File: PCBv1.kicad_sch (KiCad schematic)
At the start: 21 parts, among them J1 AVR-ISP-6, SW2 SW_Push_Reset, U1 ATmega32U4-A, Y1 16MHz

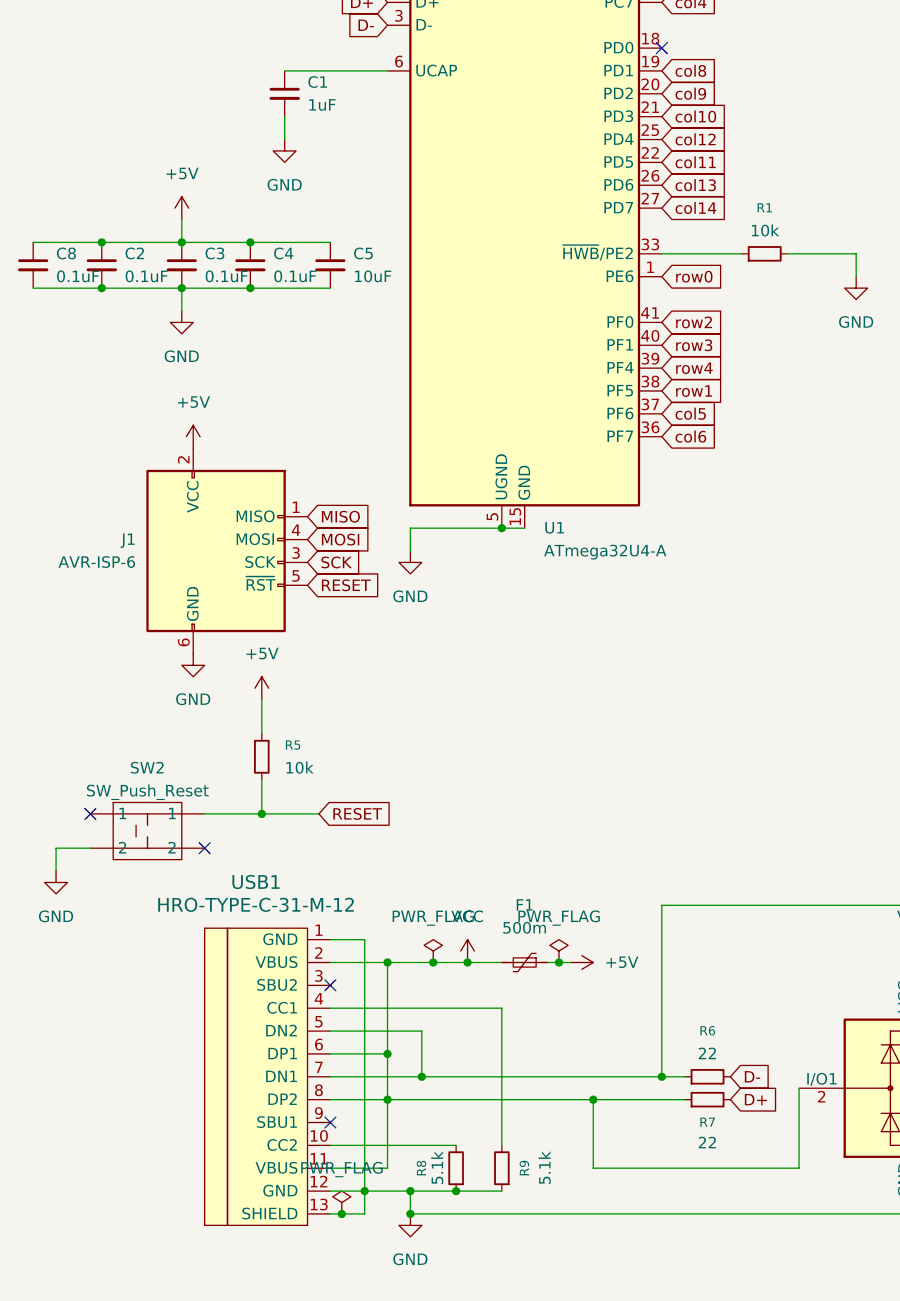
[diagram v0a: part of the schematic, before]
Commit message: maybe done but probs not
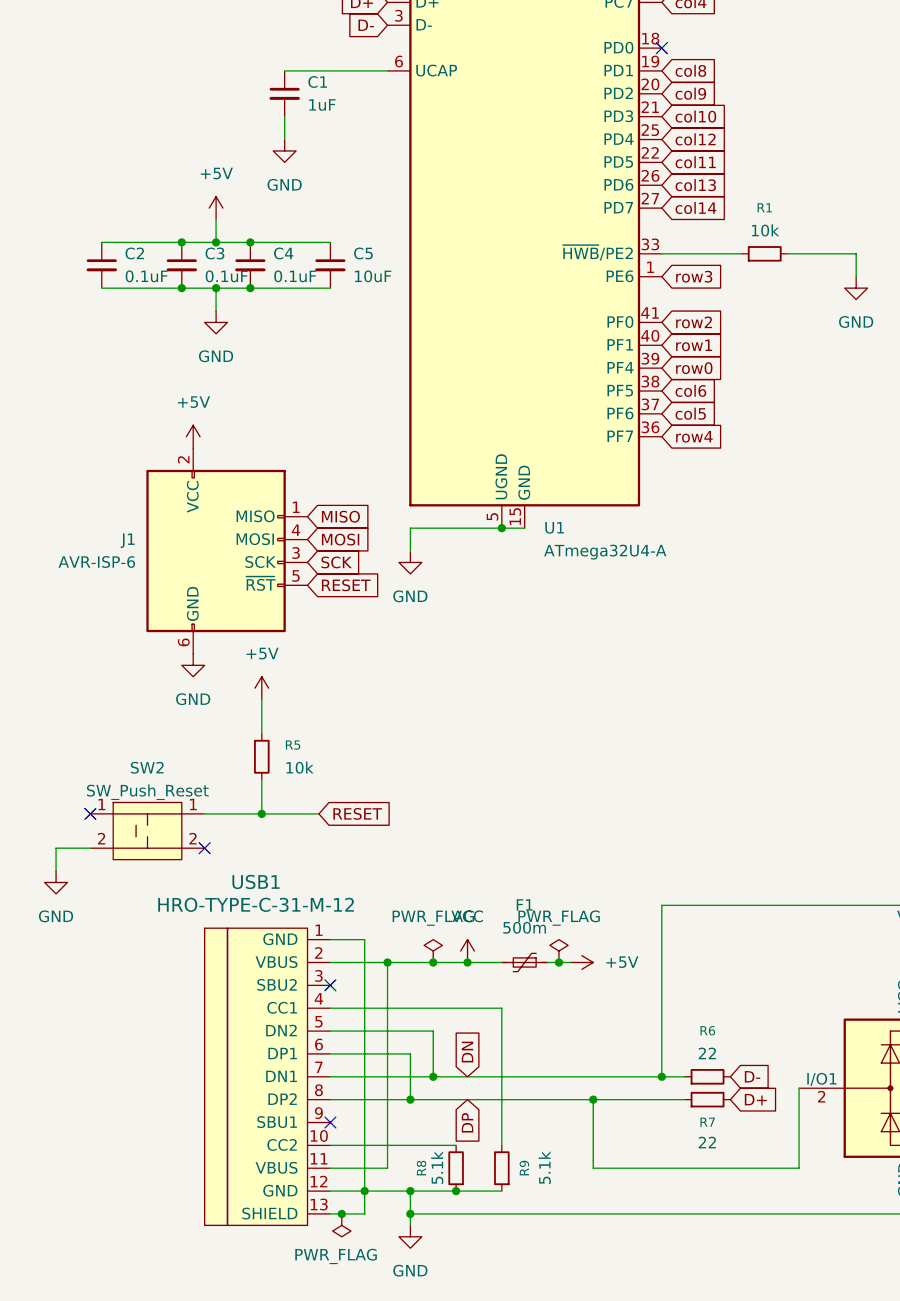
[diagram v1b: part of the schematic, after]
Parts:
- removed C8: 0.1uF, Capacitor_SMD:C_0805_2012Metric_Pad1.18x1.45mm_HandSolder, symbol Device:C_Small
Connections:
- net GND: now also SW2.2; no longer SW2. (2)
- net RESET: now also SW2.1; no longer SW2. (2)
- net VCC: no longer D1.2 (I/O1), R7.1, USB1.6 (DP1), USB1.8 (DP2)
- net col6: now also U1.38 (PF5); no longer U1.36 (PF7)
- net row0: now also U1.39 (PF4); no longer U1.1 (PE6)
- net row1: now also U1.40 (PF1); no longer U1.38 (PF5)
- net row3: now also U1.1 (PE6); no longer U1.40 (PF1)
- net row4: now also U1.36 (PF7); no longer U1.39 (PF4)
- net DN: now reaches D1.3 (I/O2), R6.1, USB1.5 (DN2), USB1.7 (DN1)
- new net DP: D1.2 (I/O1), R7.1, USB1.6 (DP1), USB1.8 (DP2)
